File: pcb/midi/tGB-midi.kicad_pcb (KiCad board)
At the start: 2 copper layers, 25.2 x 31 mm, 25 parts, among them J1 MIDI_IN, J2 MIDI_THRU, J3 MIDI_OUT, J4 IO, U1 TLP2368, U2 TC7WZ07FK

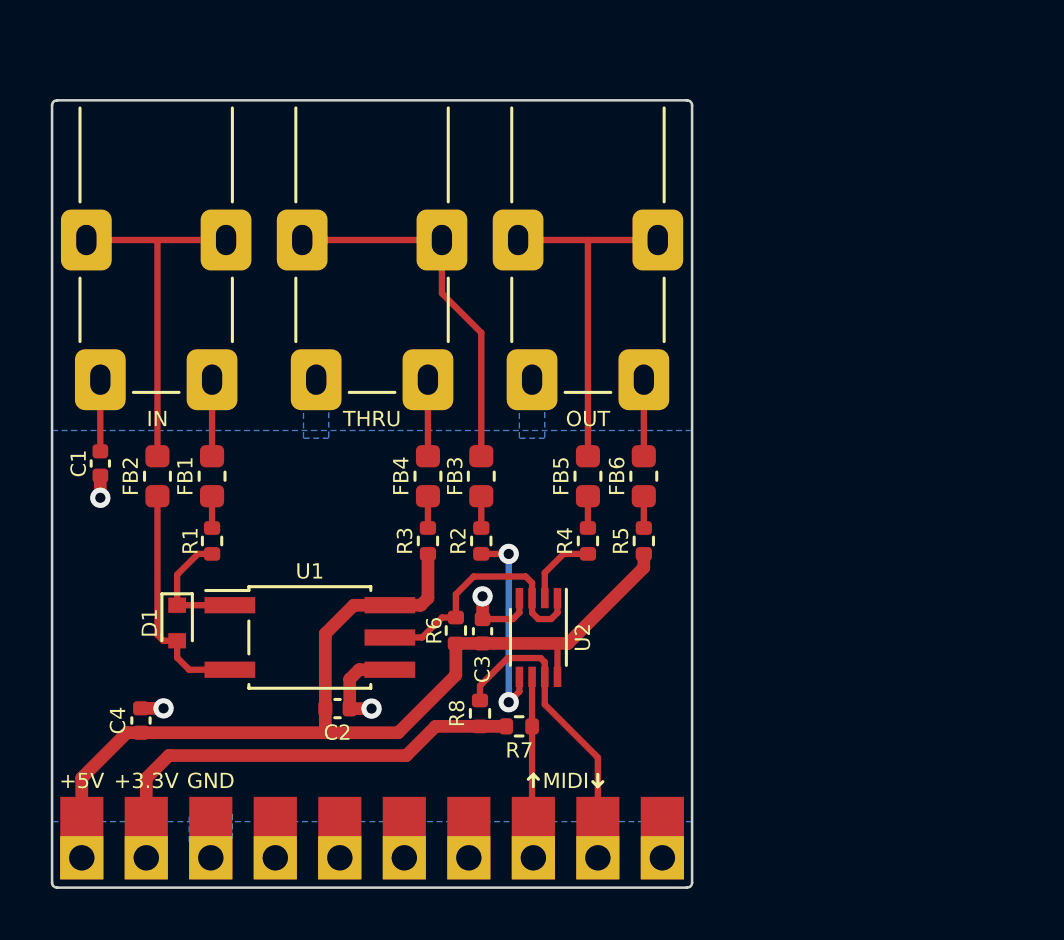
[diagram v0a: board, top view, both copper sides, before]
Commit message: update pcb (wip)
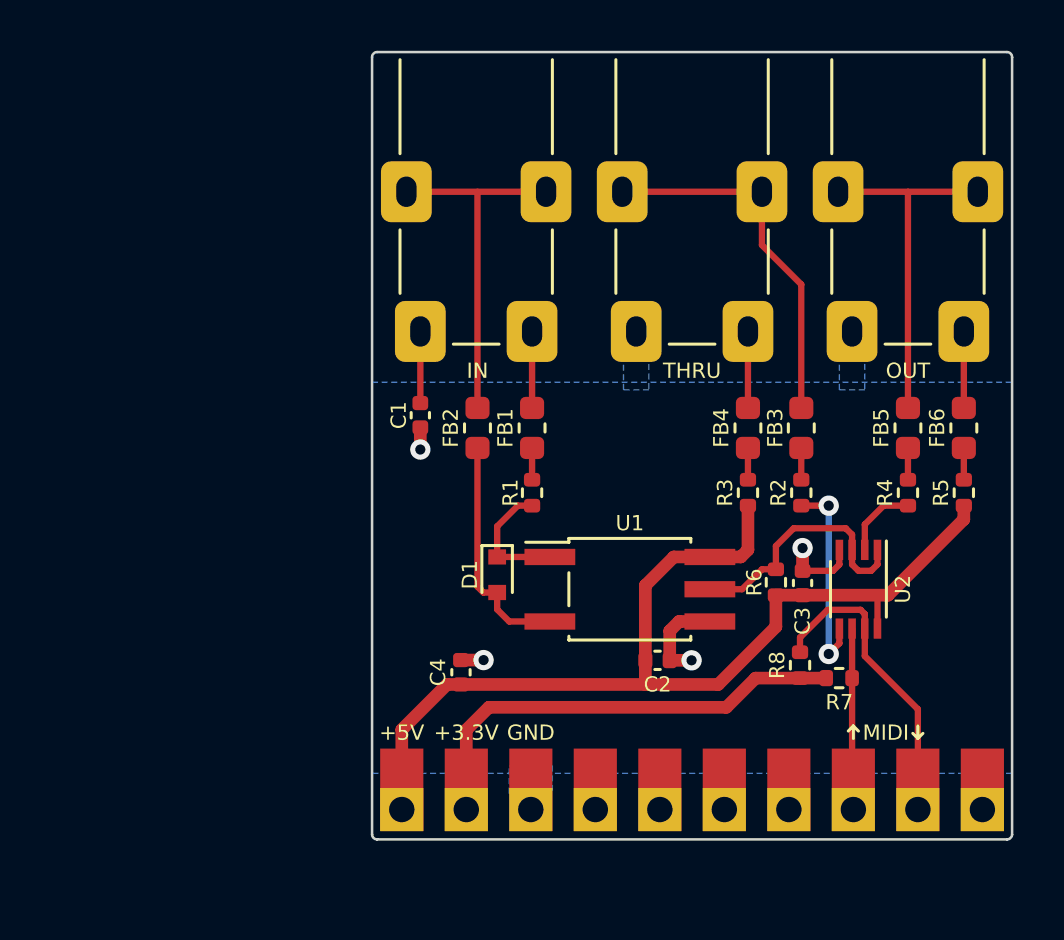
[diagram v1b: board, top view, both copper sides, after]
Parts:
- moved C3 12.7 mm to (77.0, 89.9)
- moved FB2 12.7 mm to (64.2, 83.8)
- moved FB3 12.7 mm to (76.9, 83.8)
- moved R2 12.7 mm to (76.9, 86.3)
- moved R6 12.7 mm to (75.9, 89.9)
- moved U1 12.7 mm to (70.2, 90.2)
- moved U2 12.7 mm to (79.2, 90.2)
- moved C1 12.7 mm to (61.9, 83.3)
- moved J4 12.7 mm to (61.2, 98.0)
- moved C4 12.7 mm to (63.5, 93.4)
- moved D1 12.7 mm to (64.9, 89.6)
- moved FB1 12.7 mm to (66.3, 83.8)
- moved FB4 12.7 mm to (74.8, 83.8)
- moved FB5 12.7 mm to (81.1, 83.8)
- moved FB6 12.7 mm to (83.3, 83.8)
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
